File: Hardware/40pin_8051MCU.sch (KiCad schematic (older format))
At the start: 23 parts, among them P1 CONN_10, P11 CONN_7, P2 CONN_10, P3 CONN_5X2, P4 CONN_10, P5 CONN_10, P6 CONN_9, Q1 BC557, SW1 SPST, U1 AT89S52, X1 11.0592MHz

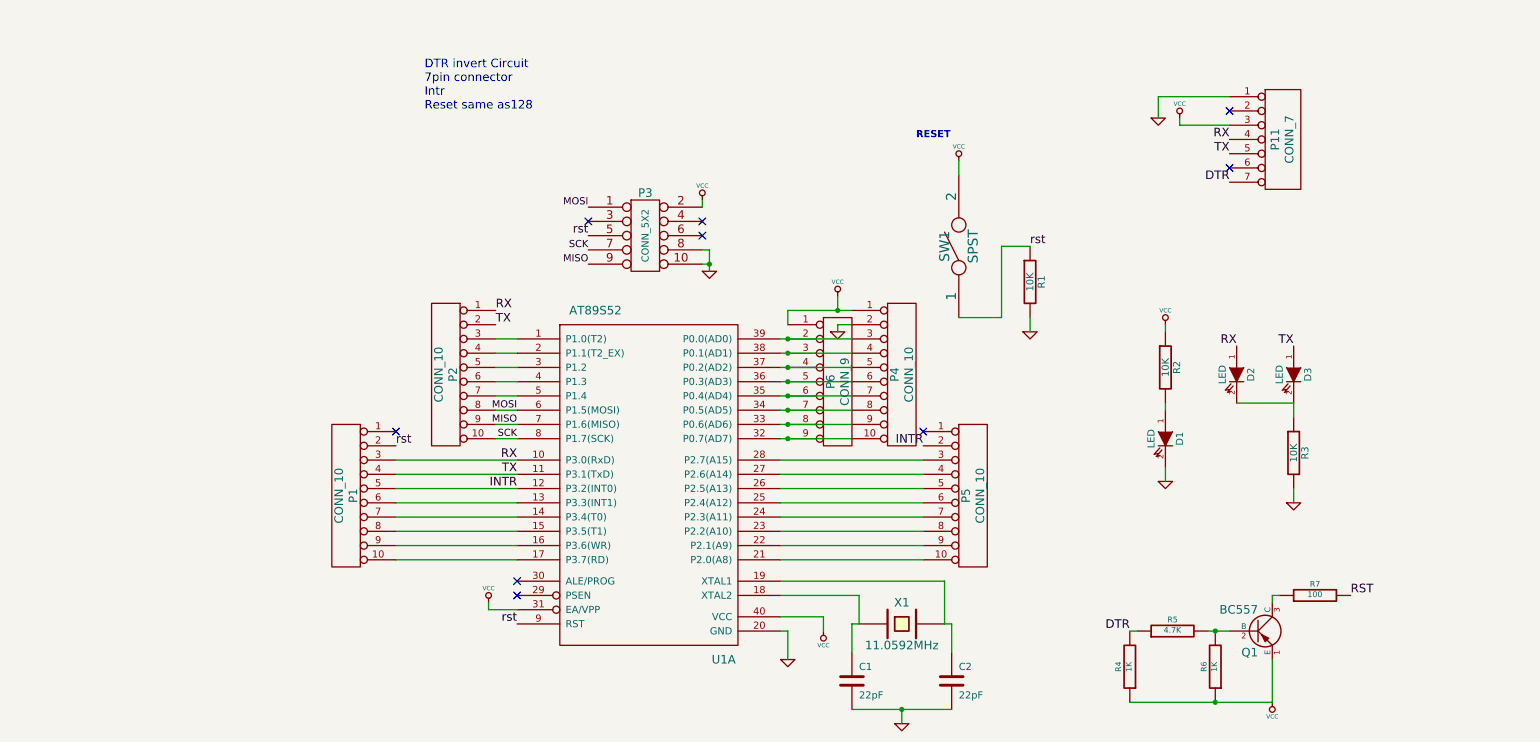
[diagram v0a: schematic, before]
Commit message: added files
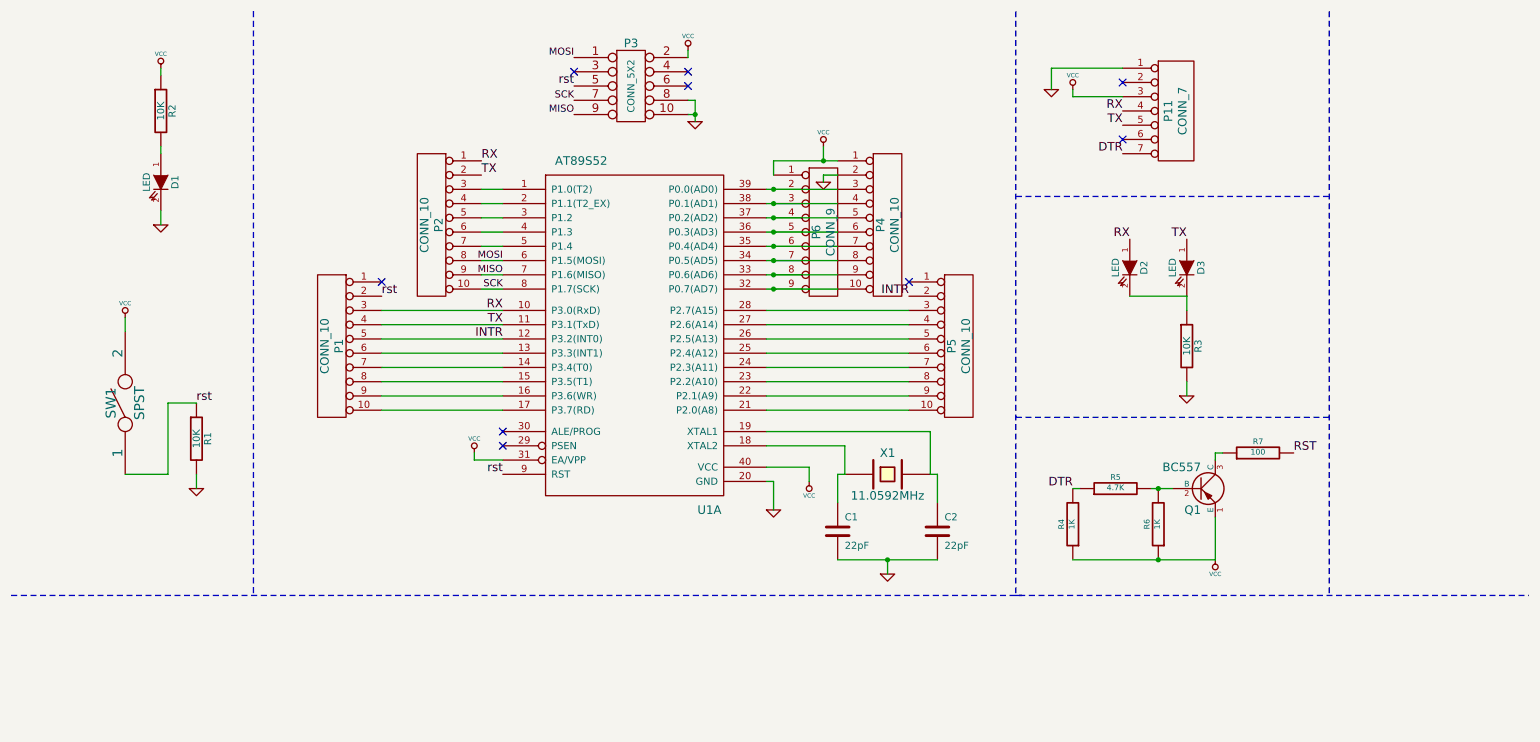
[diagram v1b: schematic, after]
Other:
- note removed: "DTR invert Circuit\n7pin connector\nIntr\nReset same as128"
- note removed: "RESET"
- moved on the sheet: C1, C2, D1, D2, D3, P1, P11, P2, P3, P4, P5, P6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
